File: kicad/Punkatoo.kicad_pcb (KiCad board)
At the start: 2 copper layers, 79 x 63.5 mm, 58 parts, among them J1 AC, J2 I/O, J3 FTDI, J4 IO 3.3v, J5 IO GND, J6 I2C, J7 Output, K1 G3MB, K2 G3MB, K3 G3MB, K4 G3MB, K5 G3MB-Relay_SolidState, Q1 BC847, Q10 BC807, Q11 BC807, Q2 BC847, Q3 BC847, Q4 BC847, Q5 BC847, Q6 BC847, Q7 BC807, Q8 BC807, Q9 BC807, SW1 Reset, SW2 Flash, U1 ESP32-WROOM-32, U2 IR RX, U3 AMS1117-3.3

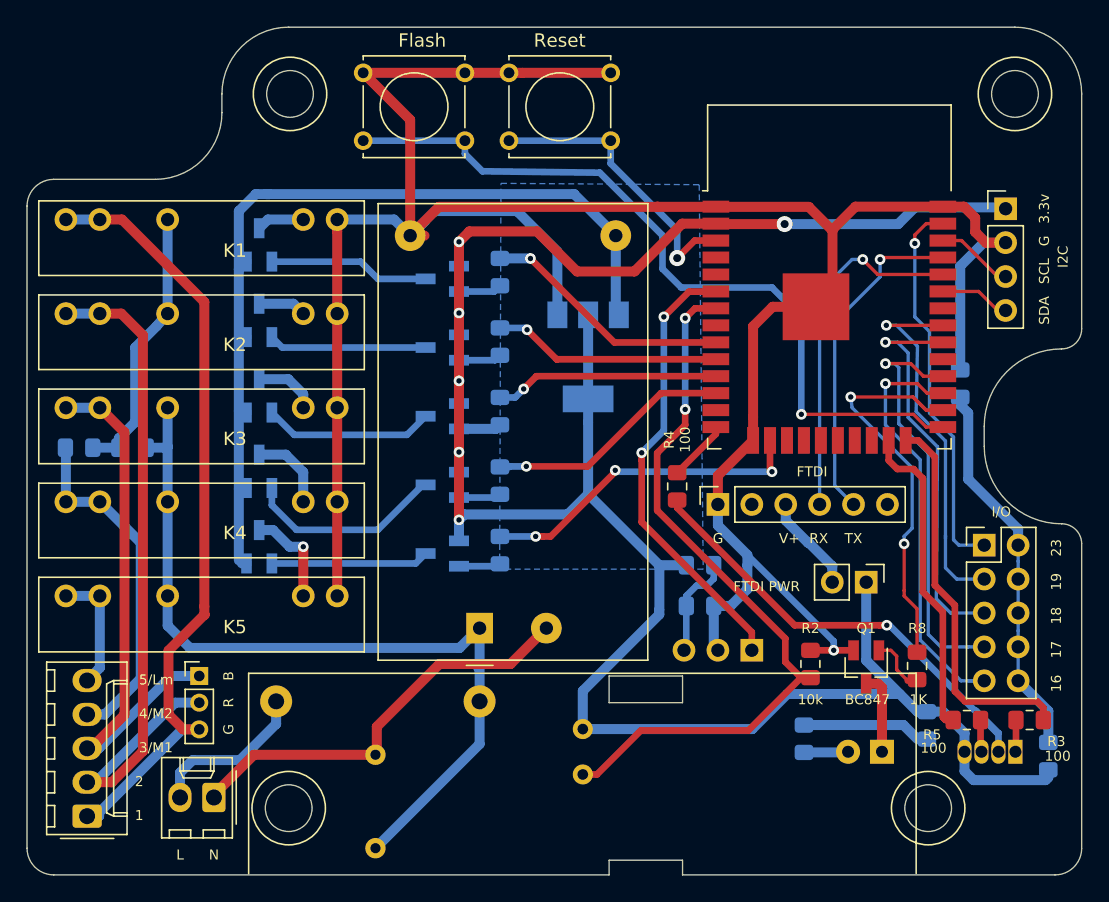
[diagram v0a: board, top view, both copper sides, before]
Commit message: ??
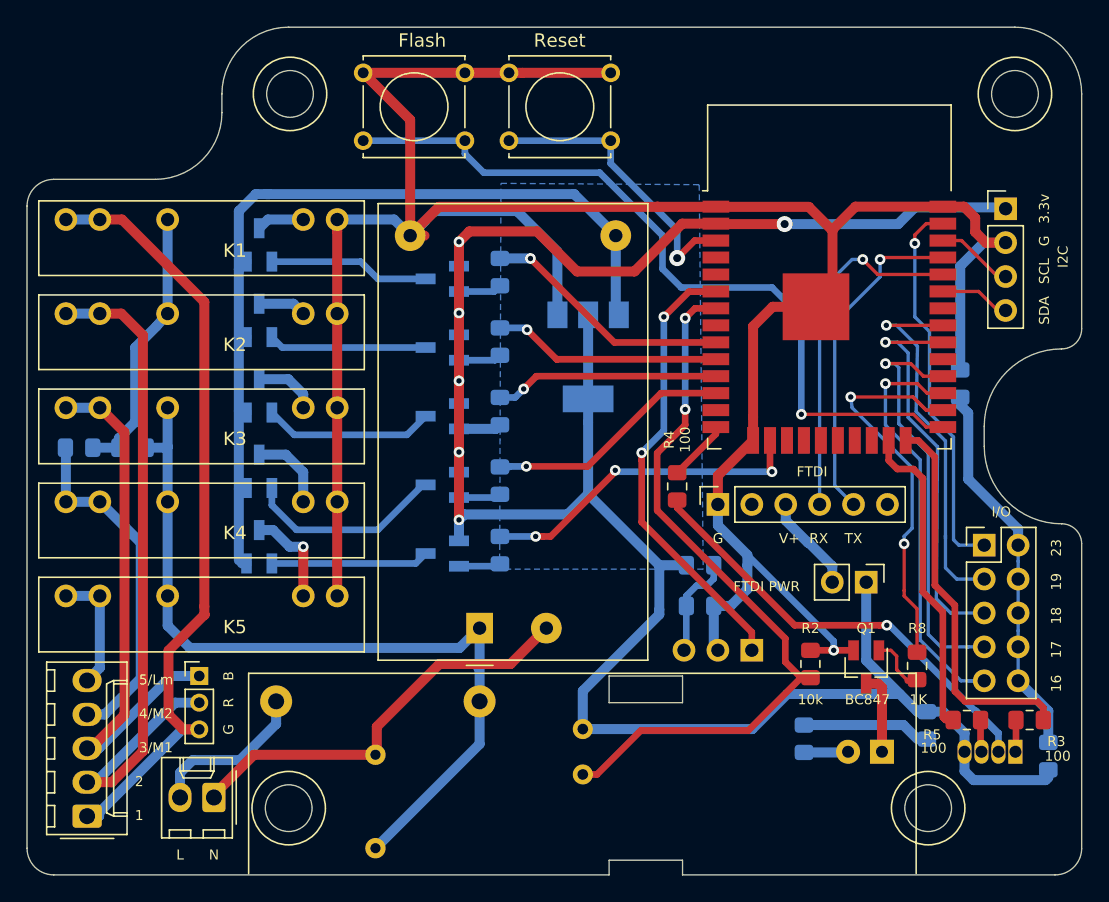
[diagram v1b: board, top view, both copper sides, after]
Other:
- net class Default removed
